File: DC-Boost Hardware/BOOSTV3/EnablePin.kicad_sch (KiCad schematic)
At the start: 2 parts

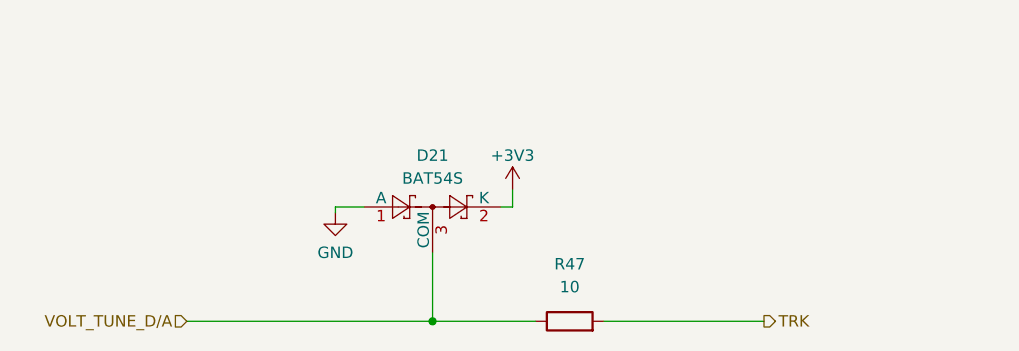
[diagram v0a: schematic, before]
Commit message: update
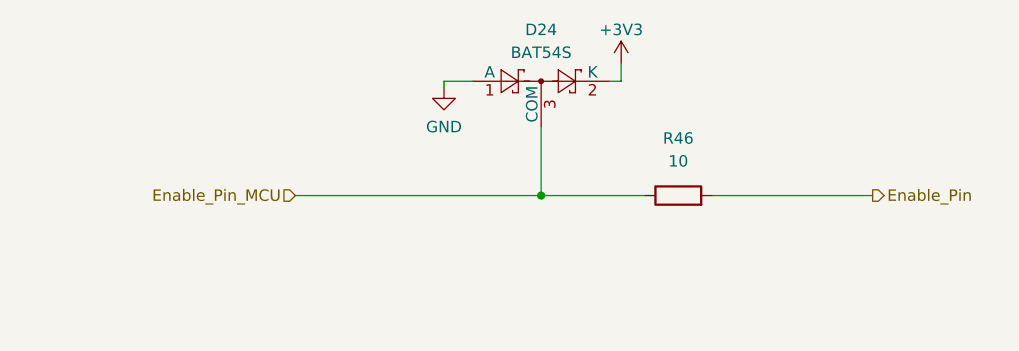
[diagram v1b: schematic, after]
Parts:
- removed D21: BAT54S, Package_TO_SOT_SMD:SOT-23, symbol Diode:BAT54S
- removed R47: 10, Resistor_SMD:R_0603_1608Metric, symbol Device:R
- added D24: BAT54S, Package_TO_SOT_SMD:SOT-23, symbol Diode:BAT54S
- added R46: 10, Resistor_SMD:R_0603_1608Metric, symbol Device:R
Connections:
- net +3V3: now also D24.2 (K)
- net GND: now also D24.1 (A)
- new net Enable_Pin: R46.2
- new net Enable_Pin_MCU: D24.3 (COM), R46.1
